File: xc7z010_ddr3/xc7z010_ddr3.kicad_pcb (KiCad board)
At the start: 2 copper layers, 100 x 100 mm, 12 parts, among them J1 SODIMM-204, U1 XC7Z010-CLG400

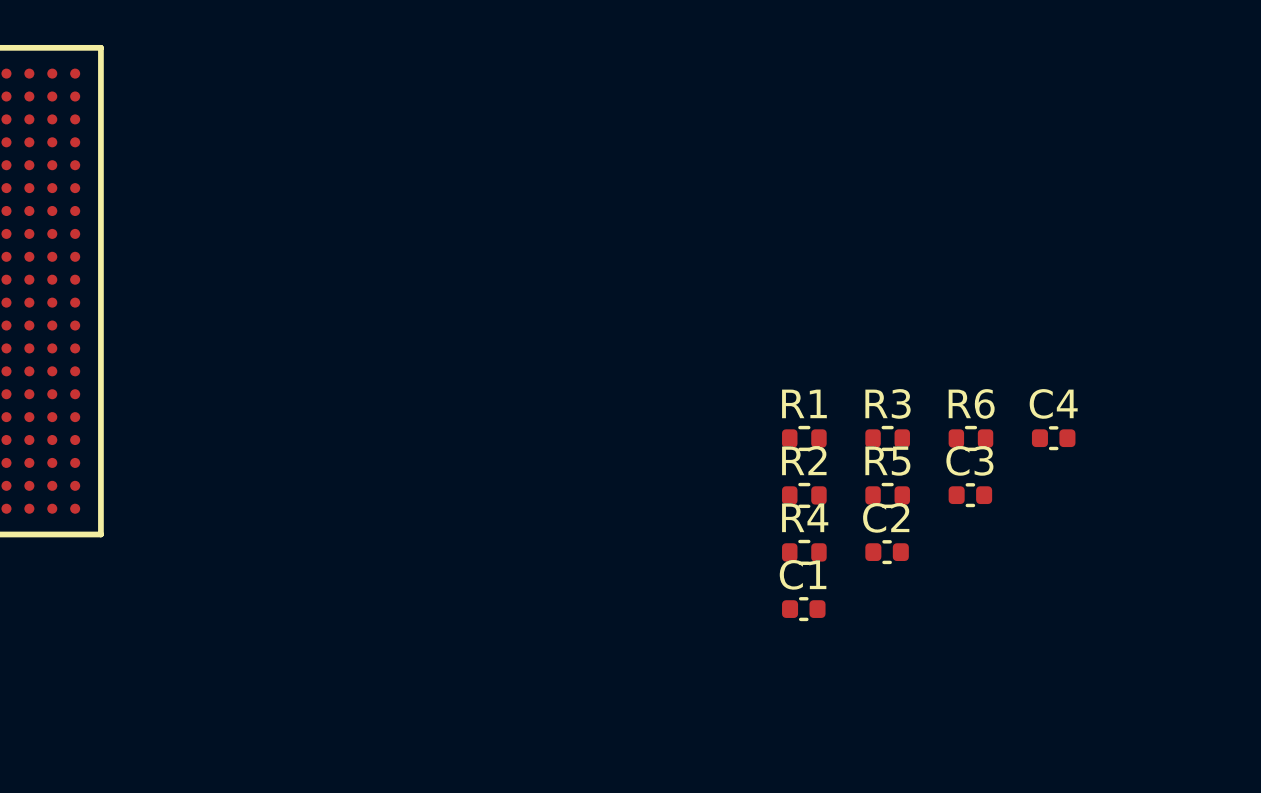
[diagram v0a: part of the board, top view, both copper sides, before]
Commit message: 202101212
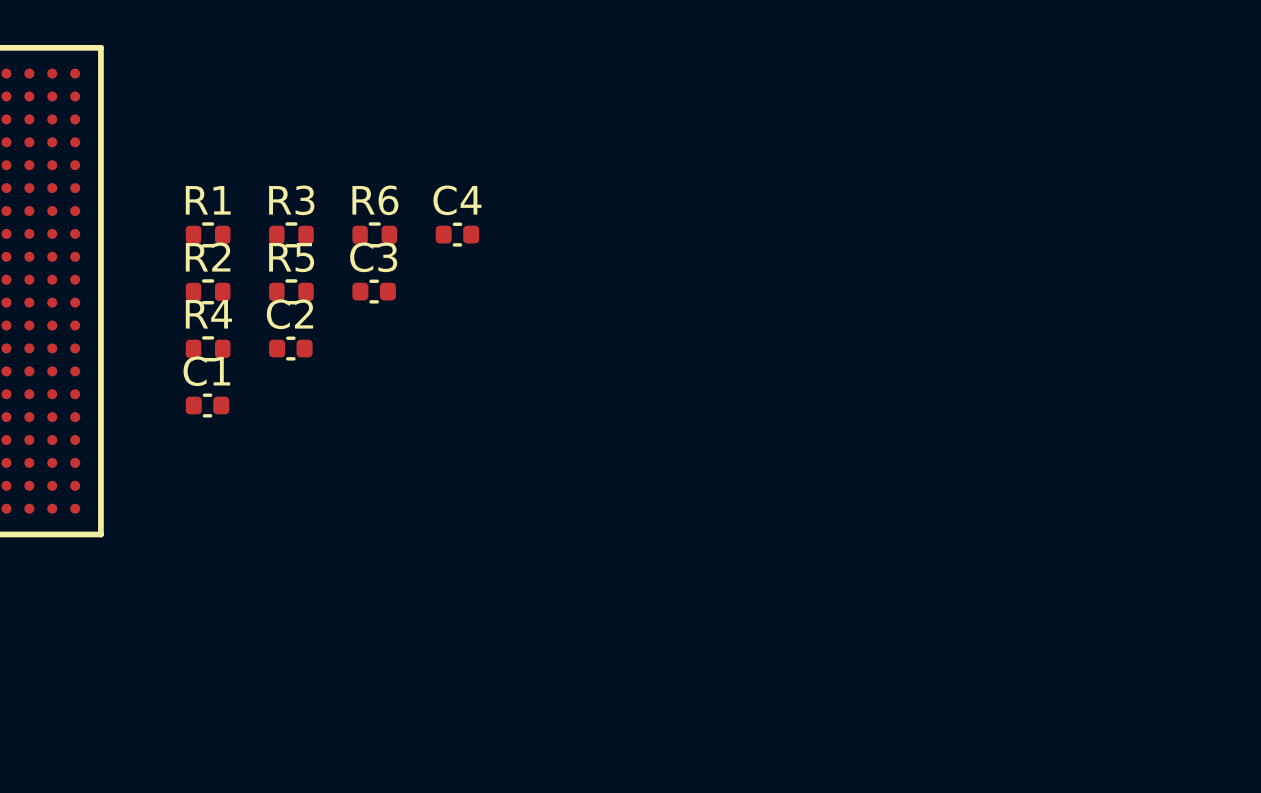
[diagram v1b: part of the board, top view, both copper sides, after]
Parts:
- moved C3 22.0 mm to (113.8, 90.8)
- moved R1 22.0 mm to (108.0, 88.8)
- moved R3 22.0 mm to (110.9, 88.8)
- moved C4 22.0 mm to (116.7, 88.8)
- moved R2 22.0 mm to (108.0, 90.8)
- moved R4 22.0 mm to (108.0, 92.8)
- moved R5 22.0 mm to (110.9, 90.8)
- moved C2 22.0 mm to (110.9, 92.8)
- moved R6 22.0 mm to (113.8, 88.8)
- moved C1 22.0 mm to (108.0, 94.7)
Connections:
- net Net-(J1-Pad101) renamed DDR_CK0_N
- net Net-(J1-Pad102) renamed DDR_CK1_P
- net Net-(J1-Pad103) renamed DDR_CK0_P
- net Net-(J1-Pad104) renamed DDR_CK1_N
- net Net-(J1-Pad114) renamed DDR_S0
- net Net-(J1-Pad120) renamed DDR_ODT1
- net Net-(J1-Pad121) renamed DDR_S1
- net Net-(J1-Pad126) renamed DDR_VREFCA
- net Net-(J1-Pad128) renamed DDR_SS
- net Net-(J1-Pad135) renamed DDR_DQS_N4
- net Net-(J1-Pad137) renamed DDR_DQS_P4
- net Net-(J1-Pad152) renamed DDR_DQS_N5
- net Net-(J1-Pad153) renamed DDR_DM5
- net Net-(J1-Pad154) renamed DDR_DQS_P5
- net Net-(J1-Pad169) renamed DDR_DQS_N6
- net Net-(J1-Pad170) renamed DDR_DM6
- net Net-(J1-Pad171) renamed DDR_DQS_P6
- net Net-(J1-Pad186) renamed DDR_DQS_N7
- net Net-(J1-Pad187) renamed DDR_DM7
- net Net-(J1-Pad188) renamed DDR_DQS_P7
- net Net-(J1-Pad197) renamed DDR_SA0
- net Net-(J1-Pad198) renamed DDR_EVENT
- net Net-(J1-Pad199) renamed DDR_VDD_SPD
- net Net-(J1-Pad200) renamed DDR_SDA
- net Net-(J1-Pad201) renamed DDR_SA1
- net Net-(J1-Pad202) renamed DDR_SCL
- net Net-(J1-Pad73) renamed DDR_CKE0
- net Net-(J1-Pad74) renamed DDR_CKE1
- J1 pad 100: Net-(J1-Pad100) -> VCC_DDR
- J1 pad 105: Net-(J1-Pad105) -> VCC_DDR
- J1 pad 106: Net-(J1-Pad106) -> VCC_DDR
- J1 pad 110: Net-(J1-Pad110) -> DDR_RAS
- J1 pad 111: Net-(J1-Pad111) -> VCC_DDR
- J1 pad 112: Net-(J1-Pad112) -> VCC_DDR
- J1 pad 113: Net-(J1-Pad113) -> DDR_WE
- J1 pad 115: Net-(J1-Pad115) -> DDR_CAS
- J1 pad 117: Net-(J1-Pad117) -> VCC_DDR
- J1 pad 118: Net-(J1-Pad118) -> VCC_DDR
- J1 pad 123: Net-(J1-Pad123) -> VCC_DDR
- J1 pad 124: Net-(J1-Pad124) -> VCC_DDR
- J1 pad 127: Net-(J1-Pad127) -> GND
- J1 pad 13: Net-(J1-Pad13) -> GND
- J1 pad 133: Net-(J1-Pad133) -> GND
- J1 pad 134: Net-(J1-Pad134) -> GND
- J1 pad 138: Net-(J1-Pad138) -> GND
- J1 pad 139: Net-(J1-Pad139) -> GND
- J1 pad 14: Net-(J1-Pad14) -> GND
- J1 pad 144: Net-(J1-Pad144) -> GND
- J1 pad 145: Net-(J1-Pad145) -> GND
- J1 pad 150: Net-(J1-Pad150) -> GND
- J1 pad 151: Net-(J1-Pad151) -> GND
- J1 pad 155: Net-(J1-Pad155) -> GND
- J1 pad 156: Net-(J1-Pad156) -> GND
- J1 pad 161: Net-(J1-Pad161) -> GND
- J1 pad 162: Net-(J1-Pad162) -> GND
- J1 pad 167: Net-(J1-Pad167) -> GND
- J1 pad 168: Net-(J1-Pad168) -> GND
- J1 pad 172: Net-(J1-Pad172) -> GND
- J1 pad 173: Net-(J1-Pad173) -> GND
- J1 pad 178: Net-(J1-Pad178) -> GND
- J1 pad 179: Net-(J1-Pad179) -> GND
- J1 pad 184: Net-(J1-Pad184) -> GND
- J1 pad 185: Net-(J1-Pad185) -> GND
- J1 pad 189: Net-(J1-Pad189) -> GND
- J1 pad 19: Net-(J1-Pad19) -> GND
- J1 pad 190: Net-(J1-Pad190) -> GND
- J1 pad 195: Net-(J1-Pad195) -> GND
- J1 pad 196: Net-(J1-Pad196) -> GND
- J1 pad 2: Net-(J1-Pad2) -> GND
- J1 pad 20: Net-(J1-Pad20) -> GND
- J1 pad 203: Net-(J1-Pad203) -> DDR_VTT
- J1 pad 204: Net-(J1-Pad204) -> DDR_VTT
- J1 pad 25: Net-(J1-Pad25) -> GND
- J1 pad 26: Net-(J1-Pad26) -> GND
- J1 pad 3: Net-(J1-Pad3) -> GND
- J1 pad 31: Net-(J1-Pad31) -> GND
- J1 pad 32: Net-(J1-Pad32) -> GND
- J1 pad 37: Net-(J1-Pad37) -> GND
- J1 pad 38: Net-(J1-Pad38) -> GND
- J1 pad 43: Net-(J1-Pad43) -> GND
- J1 pad 44: Net-(J1-Pad44) -> GND
- J1 pad 48: Net-(J1-Pad48) -> GND
- J1 pad 49: Net-(J1-Pad49) -> GND
- J1 pad 54: Net-(J1-Pad54) -> GND
- J1 pad 55: Net-(J1-Pad55) -> GND
- J1 pad 60: Net-(J1-Pad60) -> GND
- J1 pad 61: Net-(J1-Pad61) -> GND
- J1 pad 65: Net-(J1-Pad65) -> GND
- J1 pad 66: Net-(J1-Pad66) -> GND
- J1 pad 71: Net-(J1-Pad71) -> GND
- J1 pad 72: Net-(J1-Pad72) -> GND
- J1 pad 75: Net-(J1-Pad75) -> VCC_DDR
- J1 pad 76: Net-(J1-Pad76) -> VCC_DDR
- J1 pad 8: Net-(J1-Pad8) -> GND
- J1 pad 81: Net-(J1-Pad81) -> VCC_DDR
- J1 pad 82: Net-(J1-Pad82) -> VCC_DDR
- J1 pad 87: Net-(J1-Pad87) -> VCC_DDR
- J1 pad 88: Net-(J1-Pad88) -> VCC_DDR
- J1 pad 9: Net-(J1-Pad9) -> GND
- J1 pad 93: Net-(J1-Pad93) -> VCC_DDR
- J1 pad 94: Net-(J1-Pad94) -> VCC_DDR
- J1 pad 99: Net-(J1-Pad99) -> VCC_DDR
